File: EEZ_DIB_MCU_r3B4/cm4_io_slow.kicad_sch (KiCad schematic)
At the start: 6 parts, among them J3 HR911130A

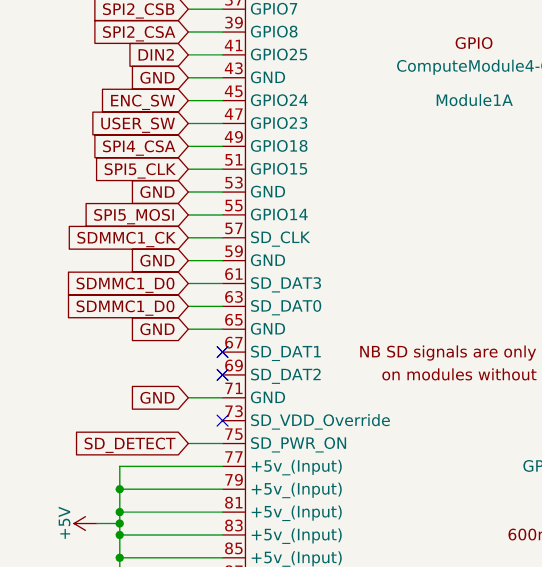
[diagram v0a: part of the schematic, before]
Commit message: Update pictures and 3D models
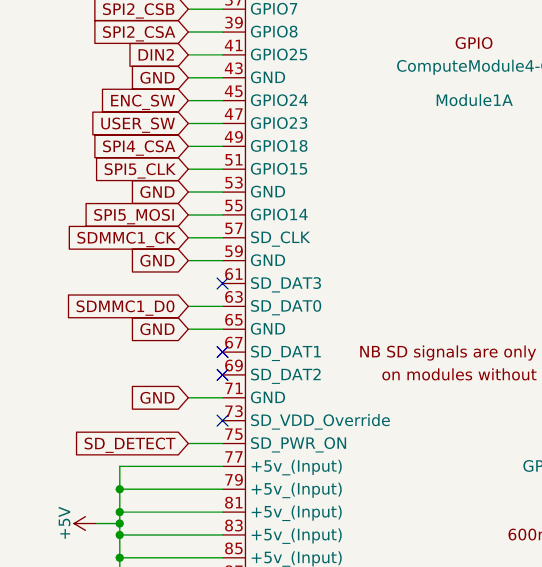
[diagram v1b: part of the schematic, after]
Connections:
- net SDMMC1_D0: no longer Module1.61 (SD_DAT3)
- no-connect marks 17 -> 18
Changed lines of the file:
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@@
   (no_connect (at 162.56 194.31))
   (no_connect (at 101.6 166.37))
+  (no_connect (at 101.6 156.21))
   (no_connect (at 162.56 100.33))
   (no_connect (at 162.56 189.23))
@@
     (stroke (width 0) (type default))
   )
-  (wire (pts (xy 101.6 156.21) (xy 97.79 156.21))
-    (stroke (width 0) (type default))
-  )
   (wire (pts (xy 101.6 146.05) (xy 97.79 146.05))
     (stroke (width 0) (type default))
@@
       (effects (font (size 1.27 1.27)) (justify right) hide)
     )
-  )
-  (global_label "SDMMC1_D0" (shape input) (at 97.79 156.21 180) (fields_autoplaced)
-    (effects (font (size 1.27 1.27)) (justify right))
-    (property "Intersheetrefs" "${INTERSHEET_REFS}" (at 83.5753 156.21 0)
-      (effects (font (size 1.27 1.27)) (justify right) hide)
-    )
